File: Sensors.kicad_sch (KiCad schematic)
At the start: 17 parts, among them U1 LPS22HH, U5 BMI270, U6 LIS3MDL, U6 NEO-M9N

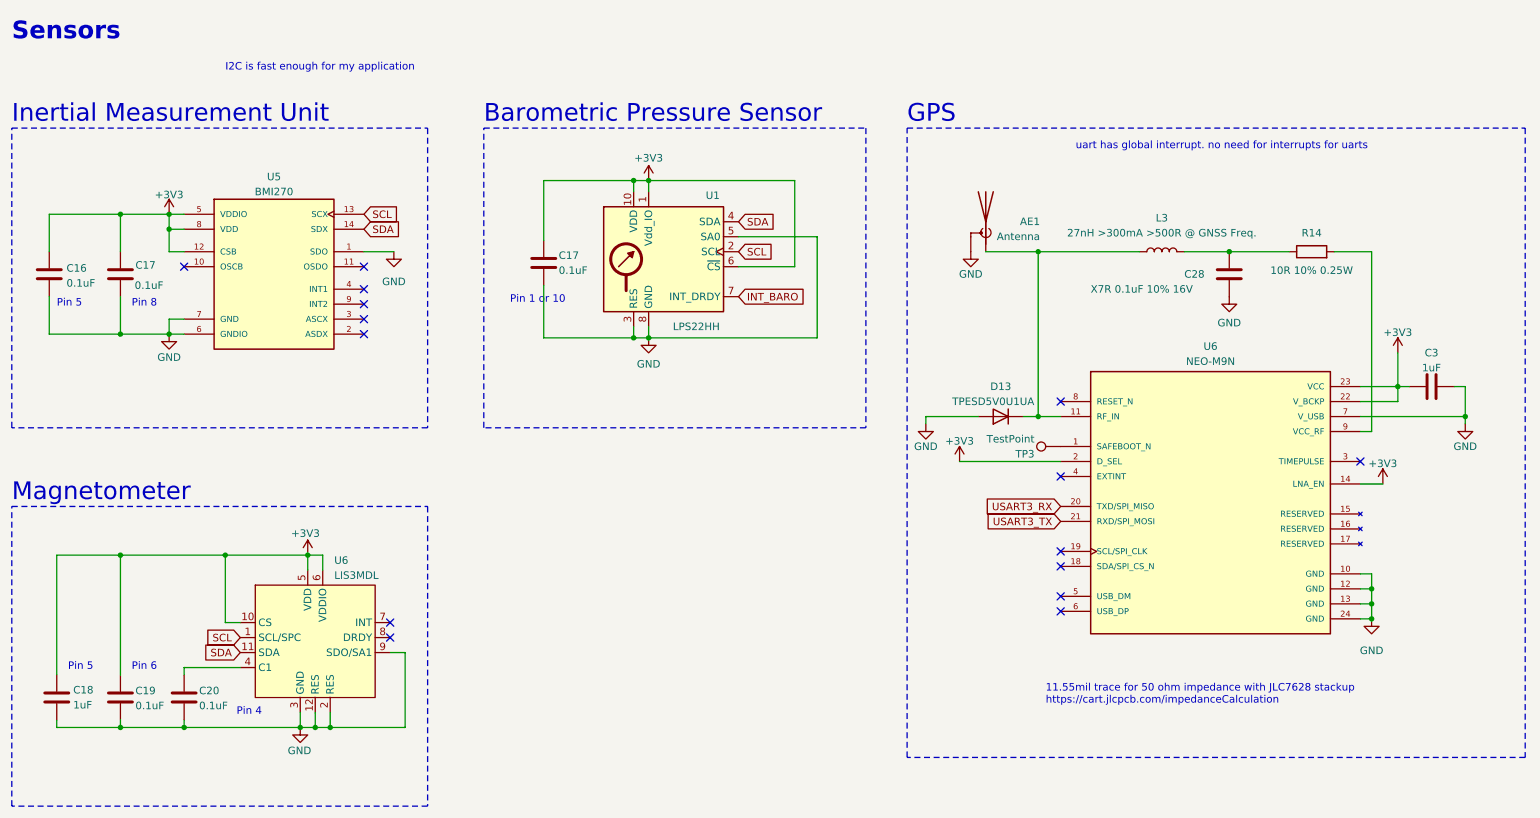
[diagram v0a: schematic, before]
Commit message: Add files via upload
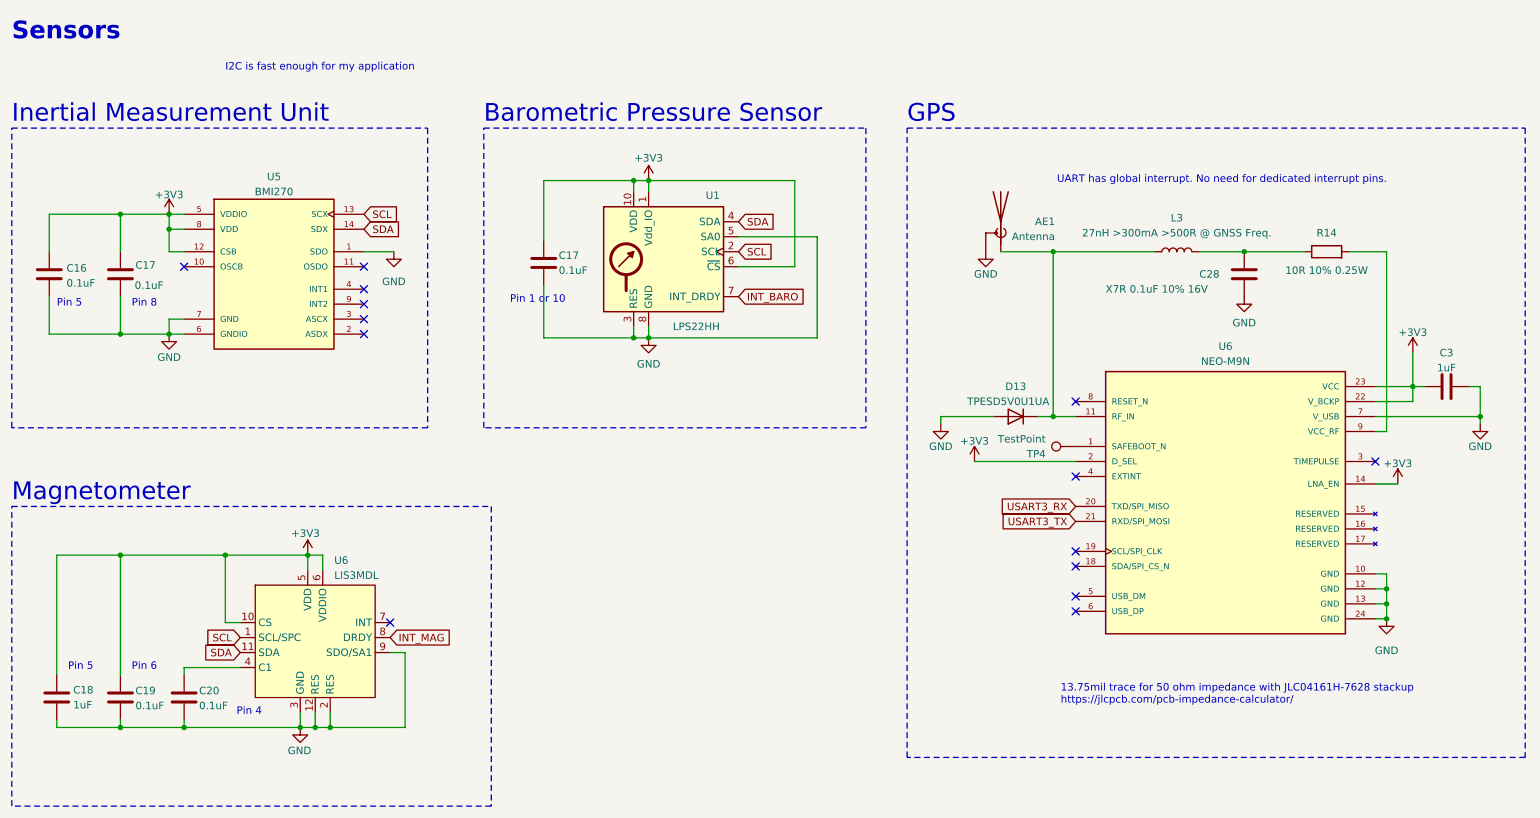
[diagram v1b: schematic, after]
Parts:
- removed TP3: TestPoint, TestPoint:TestPoint_Pad_D1.5mm, symbol Connector:TestPoint
- added TP4: TestPoint, TestPoint:TestPoint_Keystone_5000-5004_Miniature, symbol Connector:TestPoint
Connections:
- net INT_MAG: now reaches U6.8 (DRDY)
- net at U6.1 (SAFEBOOT_N): now also TP4.1
- no-connect marks 15 -> 14
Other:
- note added: "13.75mil trace for 50 ohm impedance with JLC04161H-7628 stackup https://jlcpcb.com/pcb-impedance-calculator/"
- note added: "UART has global interrupt. No need for dedicated interrupt pins."
- note removed: "11.55mil trace for 50 ohm impedance with JLC7628 stackup https://cart.jlcpcb.com/impedanceCalculation"
- note removed: "uart has global interrupt. no need for interrupts for uarts"
- moved on the sheet: AE1, C28, C3, D13, L3, R14, U6
